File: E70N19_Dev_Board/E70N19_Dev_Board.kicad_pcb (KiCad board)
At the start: 2 copper layers, 77 parts, among them J1 USB_microB_2040002-1, J2 Battery 1x2, J3 JTAGSEL_JUMPER 1x3, J4 UART_PROG 1x2, J5 ERASE_JUMPER 1x3, J6 ARM-Cortex-Debug-10, J7 CAN 1x2, J8 Conn_02x15_Counter_Clockwise, J9 Conn_02x15_Counter_Clockwise, SW1 NRST_BUTTON, U1 MCP73831, U2 TPS2112A, U3 SPX3819M5-L-3-3, U4 ATSAME70N19, U5 RT9818A-18GV, U6 SN65HVD233-Q1, Y1 Crystal_Small, Y2 Crystal

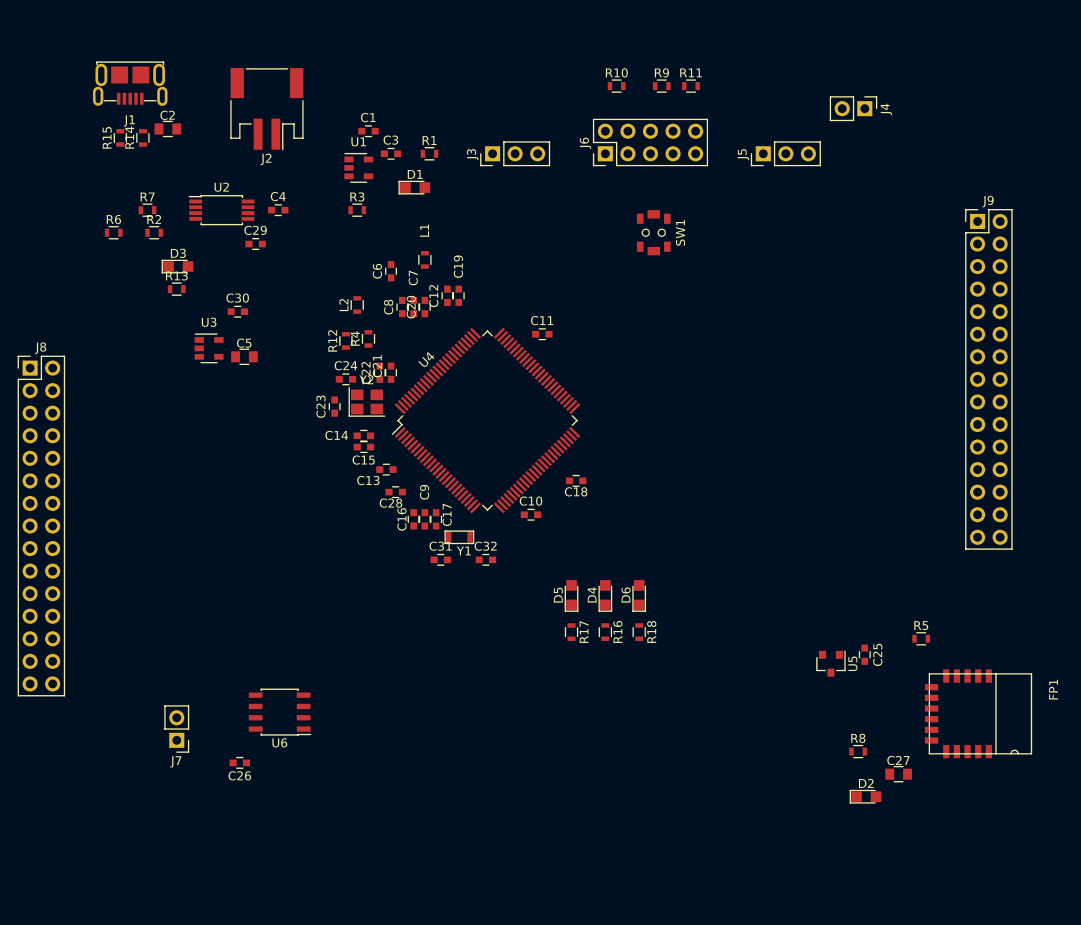
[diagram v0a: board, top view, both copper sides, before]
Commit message: Initial routing
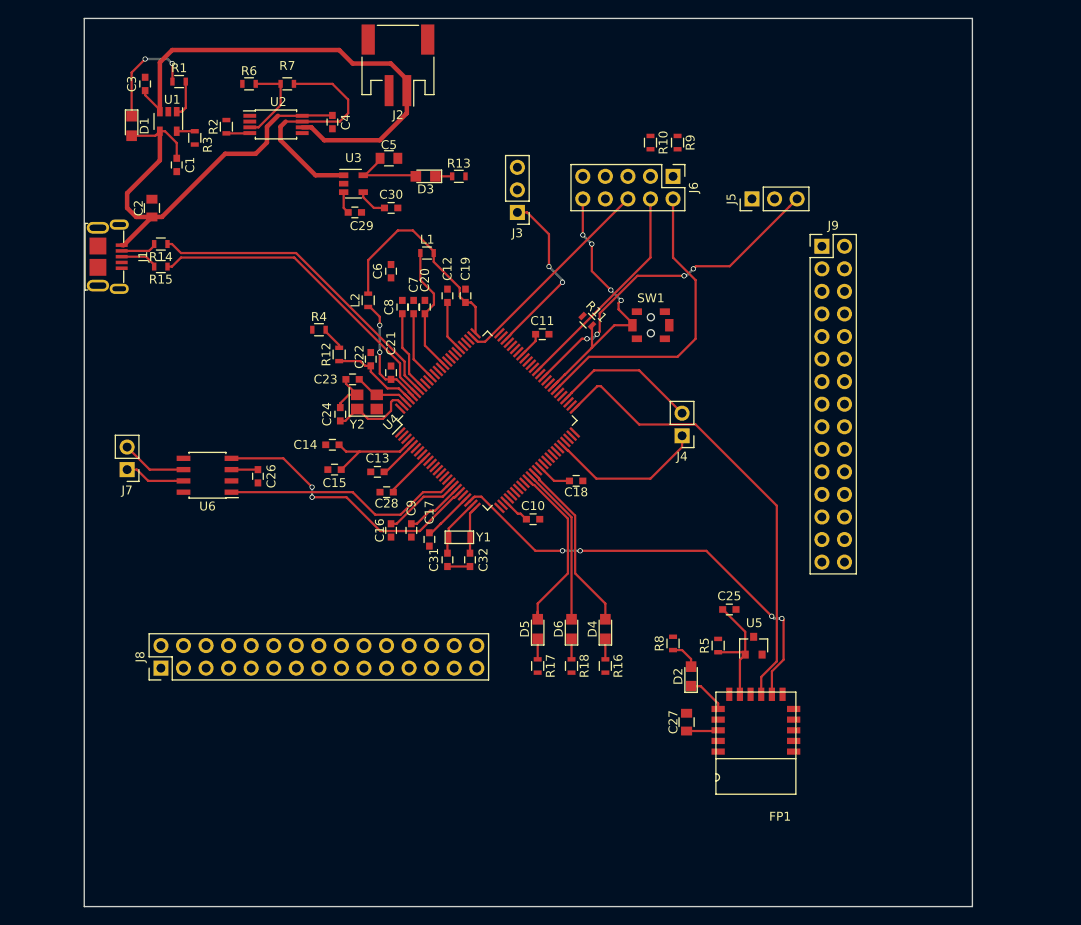
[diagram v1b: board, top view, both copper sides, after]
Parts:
- moved J4 42.2 mm to (150.9, 72.4), turned to 180 degrees
- moved J8 36.9 mm to (92.2, 98.6), turned to 90 degrees
- moved R13 34.2 mm to (125.7, 43.2)
- moved D1 32.7 mm to (88.9, 37.5), turned to 270 degrees
- moved C26 32.3 mm to (103.1, 77.0), turned to 270 degrees
- moved J7 31.0 mm to (88.4, 76.2)
- moved D3 29.6 mm to (122.0, 43.2), turned to 180 degrees
- moved R1 29.3 mm to (94.2, 32.5), turned to 180 degrees
- moved R11 28.9 mm to (140.2, 59.4), turned to 315 degrees
- moved C3 28.8 mm to (90.4, 32.8), turned to 90 degrees
- moved U6 27.9 mm to (97.4, 76.8)
- moved C5 27.6 mm to (117.9, 41.1)
- moved U3 24.7 mm to (113.9, 44.0)
- moved C27 24.6 mm to (151.4, 104.6), turned to 90 degrees
- moved R8 24.1 mm to (149.9, 95.8), turned to 270 degrees
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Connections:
- net Net-(R14-Pad1) renamed /D_N
- net Net-(R15-Pad1) renamed /D_P
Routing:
- net +3V3: track 0.00 -> 61.2 mm
- net Net-(C3-Pad1): track 0.00 -> 55.8 mm
- net Net-(C14-Pad1): track 0.00 -> 55.2 mm
- net /VBUS: track 0.00 -> 51.9 mm
- net Net-(FP1-Pad8): track 0.00 -> 51.3 mm
- net Net-(FP1-Pad7): track 0.00 -> 50.3 mm, vias 0 -> 4
- net Net-(J5-Pad3): track 0.00 -> 38.1 mm, vias 0 -> 4
- net /D_N: track 0.00 -> 36.0 mm
- net /D_P: track 0.00 -> 35.6 mm
- net /TMS: track 0.00 -> 34.9 mm
- net /NRST: track 0.00 -> 32.0 mm, vias 0 -> 4
- net /CAN_RX: track 0.00 -> 31.6 mm, vias 0 -> 2
- net Net-(C29-Pad1): track 0.00 -> 29.4 mm
- net /CAN_TX: track 0.00 -> 27.2 mm
- net /TCK: track 0.00 -> 24.7 mm
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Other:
- board outline added: 100 x 100 mm
- net class Default: trace_width 0.1524 -> 0.2032
